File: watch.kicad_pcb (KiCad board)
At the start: 4 copper layers, 38 x 38 mm, 117 parts, among them Q1 2N7002H, Q2 2N7002H, Q3 2N7002H, Q4 2N7002H, U1 STM32L071CBTx, U3 TPS63900, Y1 CR_32kHz

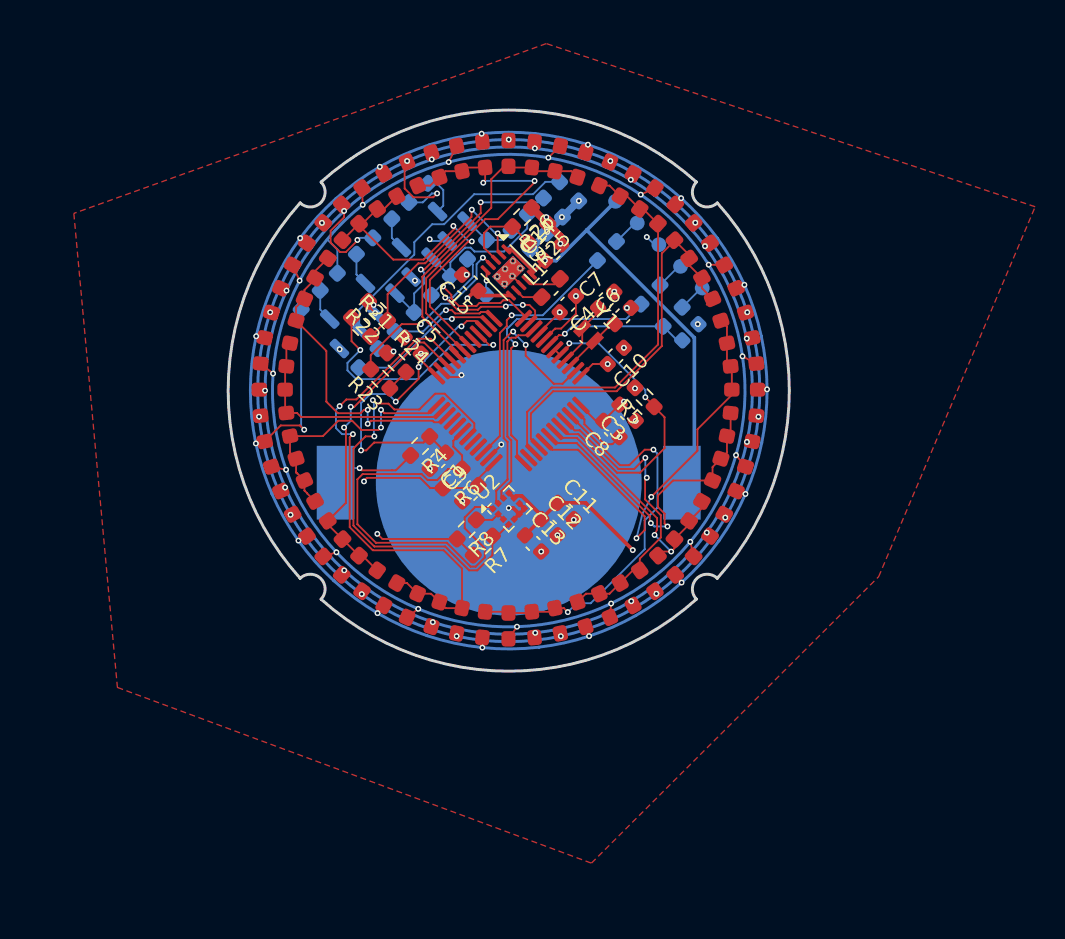
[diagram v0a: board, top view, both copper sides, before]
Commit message: ready for ordering?
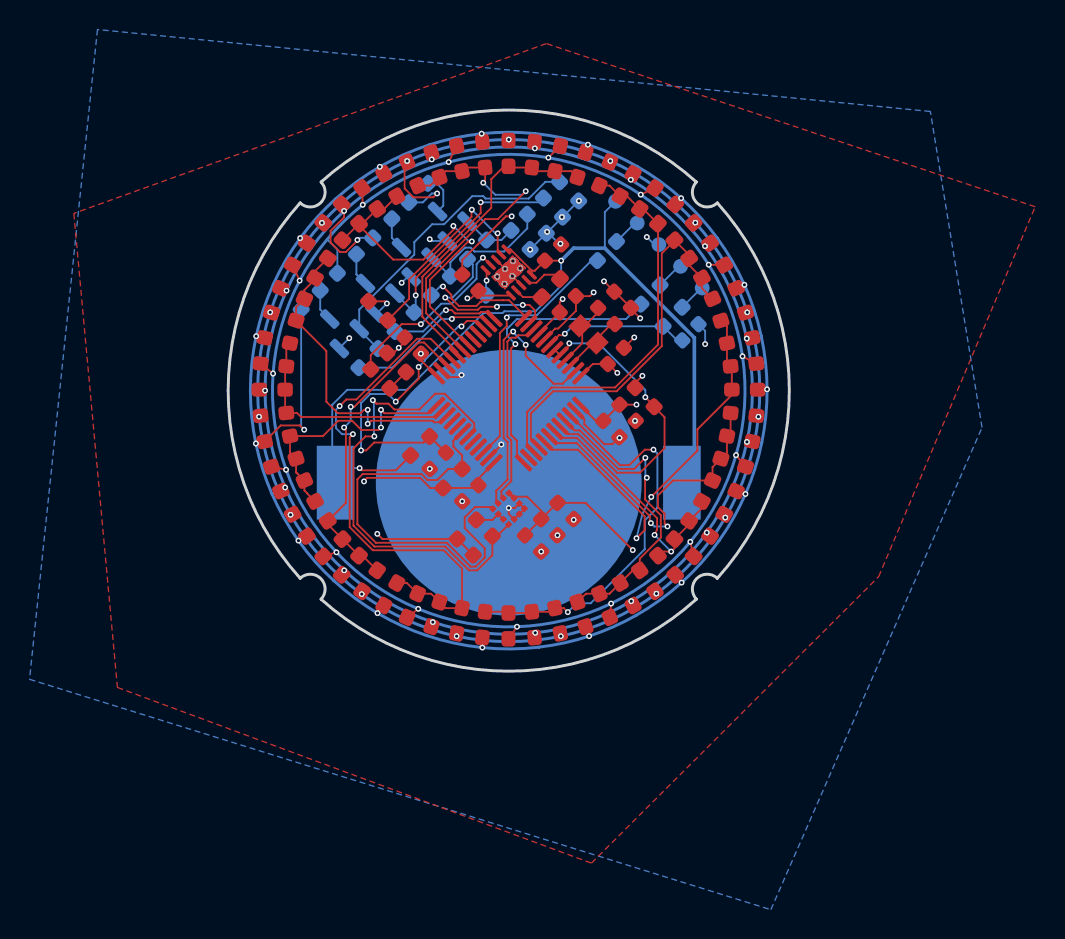
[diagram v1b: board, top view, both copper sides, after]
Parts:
- removed R21: 10K, Resistor_SMD:R_0603_1608Metric_Pad0.98x0.95mm_HandSolder
- removed R25: 39K, Resistor_SMD:R_0603_1608Metric_Pad0.98x0.95mm_HandSolder
- removed R26: 560K, Resistor_SMD:R_0603_1608Metric_Pad0.98x0.95mm_HandSolder
- R10, R11, R12, R9: value 47 -> 20
- Y1: footprint Crystal:Crystal_SMD_MicroCrystal_CM9V-T1A-2Pin_1.6x1.0mm -> Crystal:Crystal_SMD_MicroCrystal_CM9V-T1A-2Pin_1.6x1.0mm_HandSoldering
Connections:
- U1 pad 16: /Power/SEL_VDD -> unconnected-(U1-PA6-Pad16)
- U3 pad 3: Net-(U3-CFG1) -> GND
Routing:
- net +BATT: track 36.9 -> 62.3 mm
- net GND: track 30.0 -> 46.9 mm, vias 30 -> 28
- net /Power/SEL_VDD: track 16.6 -> 0.00 mm, vias 2 -> 0
- net Net-(U3-CFG1): track 5.81 -> 0.00 mm
- net VDD: track 43.3 -> 46.5 mm
- net Net-(U3-SEL): track 15.7 -> 13.9 mm
- net /LED_Matrix/LEDCOL1: track 25.7 -> 24.5 mm
- net /LED_Matrix/LEDCOL4: track 26.4 -> 25.8 mm
- added copper zone on B.Cu, net GND
